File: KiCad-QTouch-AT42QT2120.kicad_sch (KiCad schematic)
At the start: 30 parts, among them J1 Input, J2 Output, U1 AT42QT2120

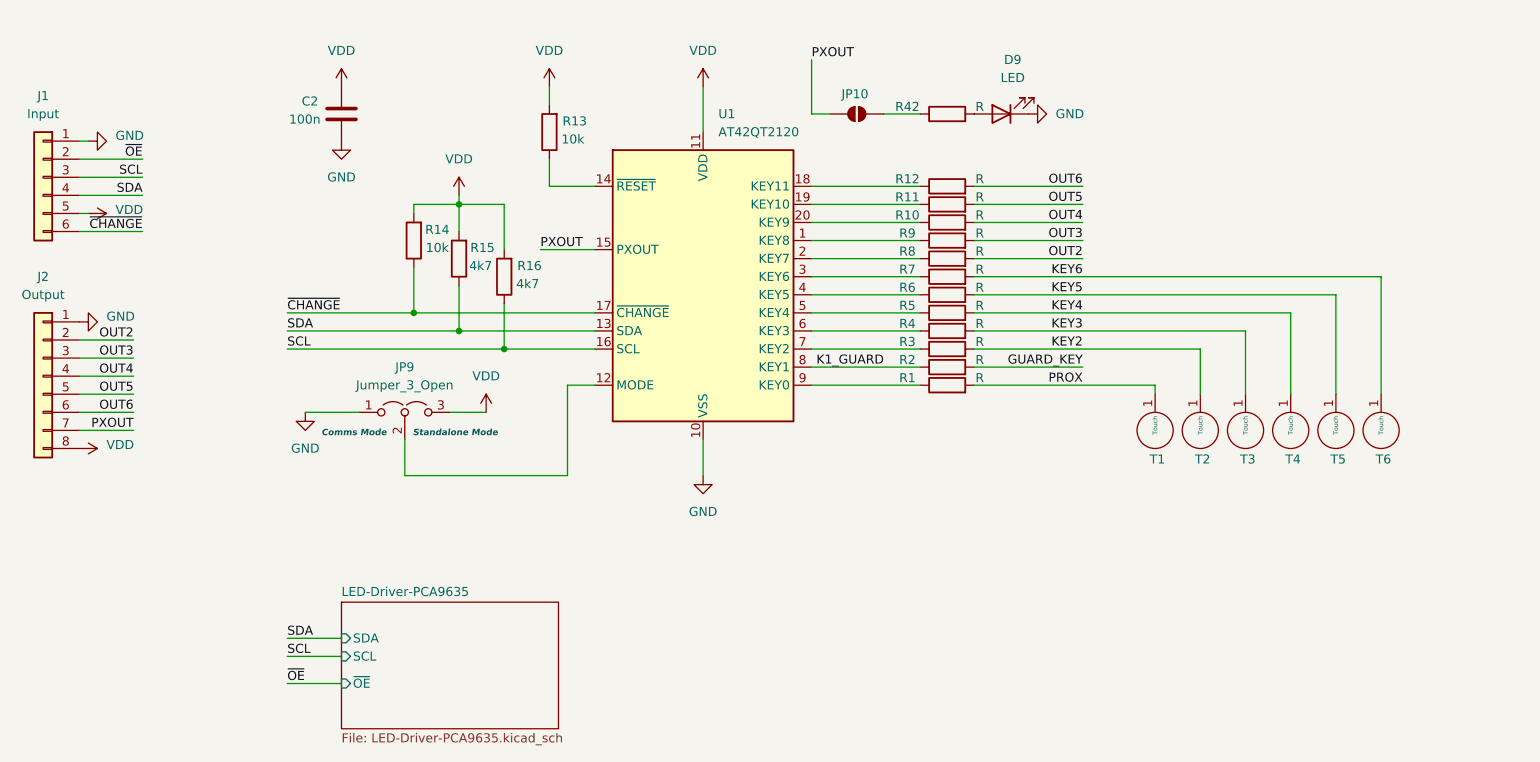
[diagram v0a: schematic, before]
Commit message: 3D rendering generation with blender
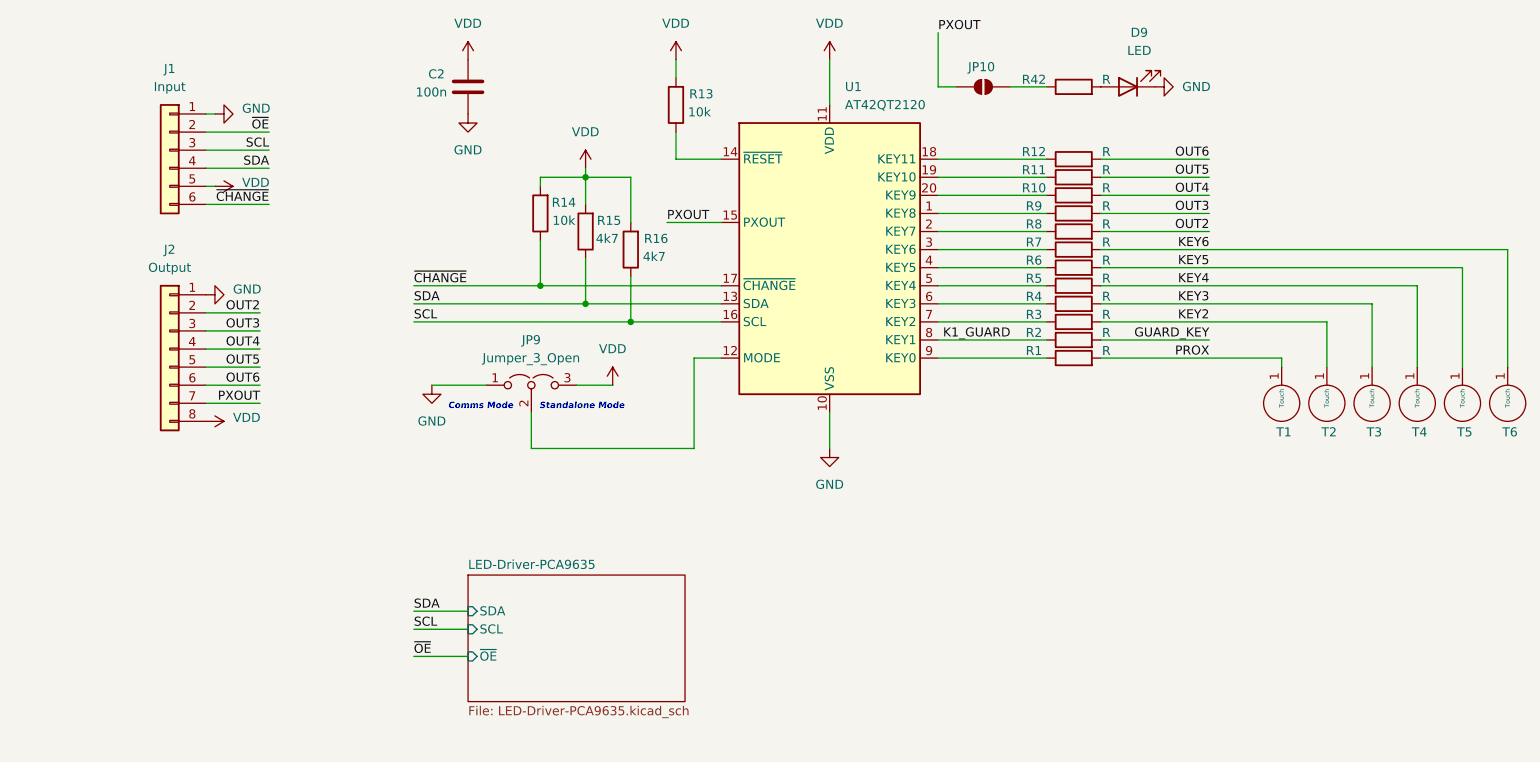
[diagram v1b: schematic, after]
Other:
- title: (none) -> Proto Board Touch-Sensor Controller
- moved on the sheet: C2, D9, J1, J2, JP10, JP9, R1, R10, R11, R12, R13, R14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
